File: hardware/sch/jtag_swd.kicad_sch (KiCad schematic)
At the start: 4 parts, among them J1 JTAG/SWD Connector

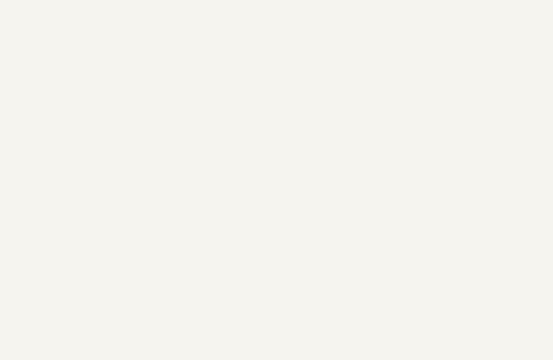
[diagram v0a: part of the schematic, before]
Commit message: USB interface half done
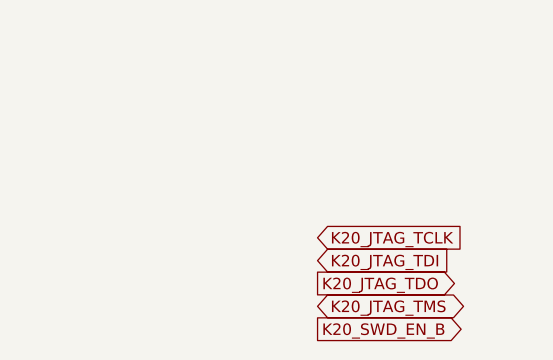
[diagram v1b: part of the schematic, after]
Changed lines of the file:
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@@
+		)
+	)
+	(global_label "K20_SWD_EN_B"
+		(shape output)
+		(at 115.57 138.43 0)
+		(fields_autoplaced yes)
+		(effects
+			(font
+				(size 1.27 1.27)
+			)
+			(justify left)
+		)
+		(property "Intersheetrefs" "${INTERSHEET_REFS}"
+			(at 132.8274 138.43 0)
+			(effects
+				(font
+					(size 1.27 1.27)
+				)
+				(justify left)
+				(hide yes)
+			)
+		)
+	)
+	(global_label "K20_JTAG_TDI"
+		(shape input)
+		(at 115.57 130.81 0)
+		(fields_autoplaced yes)
+		(effects
+			(font
+				(size 1.27 1.27)
+			)
+			(justify left)
+		)
+		(property "Intersheetrefs" "${INTERSHEET_REFS}"
+			(at 131.3156 130.81 0)
+			(effects
+				(font
+					(size 1.27 1.27)
+				)
+				(justify left)
+				(hide yes)
+			)
+		)
+	)
+	(global_label "K20_JTAG_TCLK"
+		(shape input)
+		(at 115.57 128.27 0)
+		(fields_autoplaced yes)
+		(effects
+			(font
+				(size 1.27 1.27)
+			)
+			(justify left)
+		)
+		(property "Intersheetrefs" "${INTERSHEET_REFS}"
+			(at 133.0089 128.27 0)
+			(effects
+				(font
+					(size 1.27 1.27)
+				)
+				(justify left)
+				(hide yes)
+			)
 		)
 	)
@@
 		)
 	)
+	(global_label "K20_JTAG_TDO"
+		(shape output)
+		(at 115.57 133.35 0)
+		(fields_autoplaced yes)
+		(effects
+			(font
+				(size 1.27 1.27)
+			)
+			(justify left)
+		)
+		(property "Intersheetrefs" "${INTERSHEET_REFS}"
+			(at 132.0413 133.35 0)
+			(effects
+				(font
+					(size 1.27 1.27)
+				)
+				(justify left)
+				(hide yes)
+			)
+		)
+	)
 	(global_label "KV5x_SWO{slash}TDO"
 		(shape output)
@@
 			(effects
 				(font
+					(size 1.27 1.27)
+				)
+				(justify left)
+				(hide yes)
+			)
+		)
+	)
+	(global_label "K20_JTAG_TMS"
+		(shape bidirectional)
+		(at 115.57 135.89 0)
+		(fields_autoplaced yes)
+		(effects
+			(font
+				(size 1.27 1.27)
+			)
+			(justify left)
+		)
+		(property "Intersheetrefs" "${INTERSHEET_REFS}"
+			(at 133.213 135.89 0)
+			(effects
+				(font
